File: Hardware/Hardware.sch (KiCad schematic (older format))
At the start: 1 part

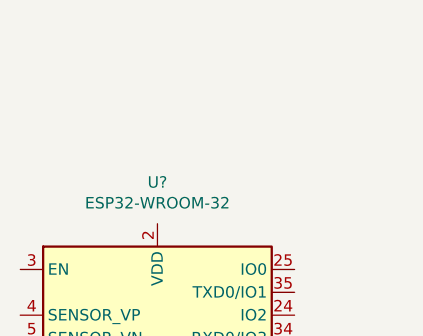
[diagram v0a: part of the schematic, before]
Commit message: Some hardware dev
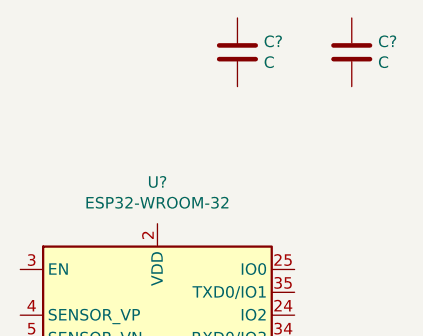
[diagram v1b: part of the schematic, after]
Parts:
- added C? (x2): C, symbol Device:C
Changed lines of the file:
@@
+	1    0    0    -1
+$EndComp
+$Comp
+L Device:C C?
+U 1 1 62087589
+P 3450 1550
+F 0 "C?" H 3565 1596 50  0000 L CNN
+F 1 "C" H 3565 1505 50  0000 L CNN
+F 2 "" H 3488 1400 50  0001 C CNN
+F 3 "~" H 3450 1550 50  0001 C CNN
+	1    3450 1550
+	1    0    0    -1
+$EndComp
+$Comp
+L Device:C C?
+U 1 1 620890B1
+P 2950 1550
+F 0 "C?" H 3065 1596 50  0000 L CNN
+F 1 "C" H 3065 1505 50  0000 L CNN
+F 2 "" H 2988 1400 50  0001 C CNN
+F 3 "~" H 2950 1550 50  0001 C CNN
+	1    2950 1550
 	1    0    0    -1
 $EndComp
